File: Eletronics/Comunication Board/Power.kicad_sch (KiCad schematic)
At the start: 8 parts, among them T1 AMS1117/3V3, U1 BATERIA

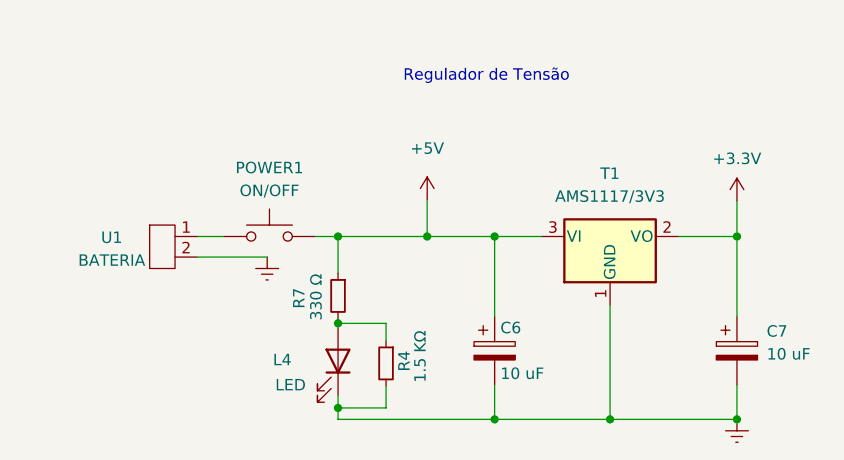
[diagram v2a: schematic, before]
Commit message: edit communication board
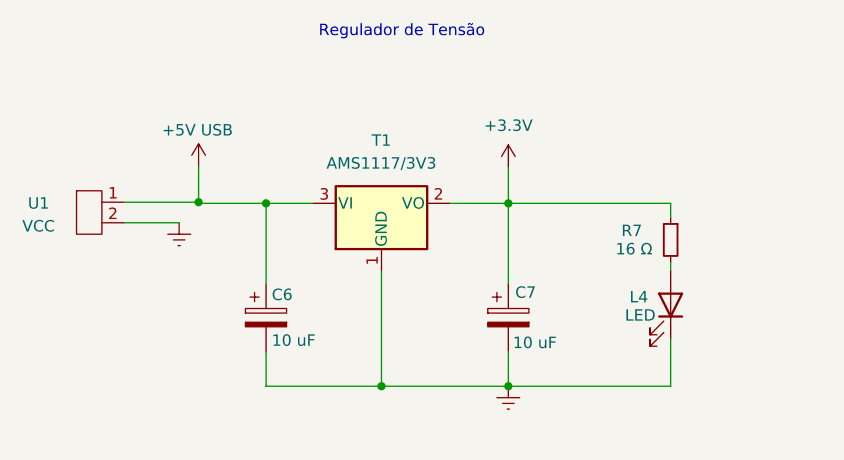
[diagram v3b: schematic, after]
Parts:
- removed POWER1: ON/OFF, Button_Switch_THT:SW_DIP_SPSTx01_Slide_6.7x4.1mm_W7.62mm_P2.54mm_LowProfile, symbol Switch:SW_Push
- removed R4: 1.5 KΩ, Resistor_SMD:R_0603_1608Metric, symbol Device:R_Small
- C6: Field5 (none) -> verificar valor
- L4: Field5 (none) -> Verificar -- outras formas -- Olhar valor do diodo se utili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
- R7: value 330 Ω -> 16 Ω
- T1: Field5 (none) -> precisa?
- U1: value BATERIA -> VCC
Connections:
- net +3.3V: now also R7.1
- net +5V USB: now reaches U1.1
- net +5V USB: now also C6.1, T1.3 (VI)
- removed net +5V: C6.1, R7.1, T1.3 (VI)
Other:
- moved on the sheet: C6, C7, L4, R7, T1, U1

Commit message: Mudanças esquematico
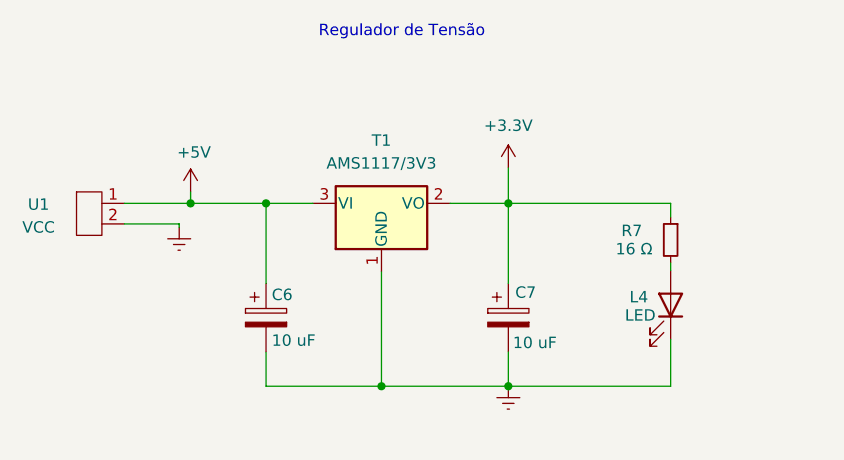
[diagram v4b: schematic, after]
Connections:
- net +5V USB renamed +5V
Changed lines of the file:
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@@
-	)
-	(junction
-		(at 114.681 92.583)
-		(diameter 0)
-		(color 0 0 0 0)
 	)
 	(junction
@@
 		(color 0 0 0 0)
 	)
-	(wire
-		(pts
-			(xy 106.426 94.869) (xy 112.522 94.869)
+	(junction
+		(at 113.792 92.71)
+		(diameter 0)
+		(color 0 0 0 0)
+	)
+	(wire
+		(pts
+			(xy 106.426 94.996) (xy 112.522 94.996)
 		)
 		(stroke
@@
 	(wire
 		(pts
+			(xy 112.522 94.996) (xy 112.522 95.377)
+		)
+		(stroke
+			(width 0)
+			(type default)
+		)
+	)
+	(wire
+		(pts
 			(xy 167.132 107.823) (xy 167.132 113.03)
 		)
@@
 	(wire
 		(pts
-			(xy 114.681 92.583) (xy 114.681 92.71)
+			(xy 113.792 91.44) (xy 113.792 92.71)
 		)
 		(stroke
@@
 	(wire
 		(pts
-			(xy 114.681 92.71) (xy 122.174 92.71)
+			(xy 113.792 92.71) (xy 122.174 92.71)
 		)
 		(stroke
@@
 	(wire
 		(pts
-			(xy 114.681 88.646) (xy 114.681 92.583)
-		)
-		(stroke
-			(width 0)
-			(type default)
-		)
-	)
-	(wire
-		(pts
-			(xy 106.426 92.583) (xy 114.681 92.583)
+			(xy 106.426 92.71) (xy 113.792 92.71)
 		)
 		(stroke
@@
 			)
 			(justify left bottom)
-		)
-	)
-	(symbol
-		(lib_id "power:+5V")
-		(at 114.681 88.646 0)
-		(unit 1)
-		(exclude_from_sim no)
-		(in_bom yes)
-		(on_board yes)
-		(dnp no)
-		(property "Reference" "#PWR0127"
-			(at 114.681 92.456 0)
-			(effects
-				(font
-					(size 1.27 1.27)
-				)
-				(hide yes)
-			)
-		)
-		(property "Value" "+5V USB"
-			(at 114.554 84.582 0)
-			(effects
-				(font
-					(size 1.27 1.27)
-				)
-			)
-		)
-		(property "Footprint" ""
-			(at 114.681 88.646 0)
-			(effects
-				(font
-					(size 1.27 1.27)
-				)
-				(hide yes)
-			)
-		)
-		(property "Datasheet" ""
-			(at 114.681 88.646 0)
-			(effects
-				(font
-					(size 1.27 1.27)
-				)
-				(hide yes)
-			)
-		)
-		(property "Description" ""
-			(at 114.681 88.646 0)
-			(effects
-				(font
-					(size 1.27 1.27)
-				)
-				(hide yes)
-			)
-		)
-		(pin "1"
-		)
-		(instances
-			(project "Comunication Board"
-				(path "/4c7888e1-33c4-4d9e-9379-8d84ea02e710/5ed939b2-ef8e-49b6-ba2b-f1c3d3dd1fd8"
-					(reference "#PWR0127")
-					(unit 1)
-				)
-			)
 		)
 	)
@@
 	)
 	(symbol
+		(lib_id "power:+5V")
+		(at 113.792 91.44 0)
+		(unit 1)
+		(exclude_from_sim no)
+		(in_bom yes)
+		(on_board yes)
+		(dnp no)
+		(property "Reference" "#PWR01"
+			(at 113.792 95.25 0)
+			(effects
+				(font
+					(size 1.27 1.27)
+				)
+				(hide yes)
+			)
+		)
+		(property "Value" "+5V"
+			(at 114.173 87.0458 0)
+			(effects
+				(font
+					(size 1.27 1.27)
+				)
+			)
+		)
+		(property "Footprint" ""
+			(at 113.792 91.44 0)
+			(effects
+				(font
+					(size 1.27 1.27)
+				)
+				(hide yes)
+			)
+		)
+		(property "Datasheet" ""
+			(at 113.792 91.44 0)
+			(effects
+				(font
+					(size 1.27 1.27)
+				)
+				(hide yes)
+			)
+		)
+		(property "Description" ""
+			(at 113.792 91.44 0)
+			(effects
+				(font
+					(size 1.27 1.27)
+				)
+				(hide yes)
+			)
+		)
+		(pin "1"
+		)
+		(instances
+			(project "Comunication Board"
+				(path "/4c7888e1-33c4-4d9e-9379-8d84ea02e710/5ed939b2-ef8e-49b6-ba2b-f1c3d3dd1fd8"
+					(reference "#PWR01")
+					(unit 1)
+				)
+			)
+		)
+	)
+	(symbol
 		(lib_id "Device:LED")
 		(at 167.132 104.013 270)
@@
 		(lib_name "BATERIA_1")
 		(lib_id "New_Library:BATERIA")
-		(at 106.426 92.837 0)
+		(at 106.426 92.964 0)
 		(unit 1)
 		(exclude_from_sim no)
@@
 		(dnp no)
 		(property "Reference" "U1"
-			(at 96.901 92.71 0)
+			(at 96.901 92.837 0)
 			(effects
 				(font
@@
 		)
 		(property "Value" "VCC"
-			(at 96.901 95.25 0)
+			(at 96.901 95.377 0)
 			(effects
 				(font
@@
 		)
 		(property "Footprint" "Connector_JST:JST_XH_B2B-XH-AM_1x02_P2.50mm_Vertical"
-			(at 102.8192 90.2716 0)
+			(at 102.8192 90.3986 0)
 			(effects
 				(font
@@
 		)
 		(property "Datasheet" ""
-			(at 102.8192 90.2716 0)
-			(effects
-				(font
-					(size 1.27 1.27)
-				)
-				(hide yes)
-			)
-		)
-		(property "Description" ""
-			(at 106.426 92.837 0)
+			(at 102.8192 90.3986 0)
+			(effects
+				(font
+					(size 1.27 1.27)
+				)
+				(hide yes)
+			)
+		)
+		(property "Description" ""
+			(at 106.426 92.964 0)
 			(effects
 				(font
@@
 	(symbol
 		(lib_id "power:GNDREF")
-		(at 112.522 94.869 0)
+		(at 112.522 95.377 0)
 		(unit 1)
 		(exclude_from_sim no)
@@
 		(fields_autoplaced yes)
 		(property "Reference" "#PWR0124"
-			(at 112.522 101.219 0)
+			(at 112.522 101.727 0)
 			(effects
 				(font
@@
 		)
 		(property "Value" "GNDREF"
-			(at 112.522 99.695 0)
+			(at 112.522 100.203 0)
 			(effects
 				(font
@@
 		)
 		(property "Footprint" ""
-			(at 112.522 94.869 0)
+			(at 112.522 95.377 0)
 			(effects
 				(font
@@
 		)
 		(property "Datasheet" ""
-			(at 112.522 94.869 0)
-			(effects
-				(font
-					(size 1.27 1.27)
-				)
-				(hide yes)
-			)
-		)
-		(property "Description" ""
-			(at 112.522 94.869 0)
-			(effects
-				(font
+			(at 112.522 95.377 0)
+			(effects
+				(font
+					(size 1.27 1.27)
+				)
+				(hide yes)
+			)
+		)
+		(property "Description" ""
+			(at 112.522 95.377 0)
+			(effects
+				(font
